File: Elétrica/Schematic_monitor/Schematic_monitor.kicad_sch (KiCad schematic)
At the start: 59 parts, among them J1 Conn_01x04, J2 USB_B_Micro, J3 Eletrode 1, J4 Eletrode 2, J5 Conn_01x09, SW1 SW_Push, SW2 SW_SPDT, U1 STM32F446RET6TR, U2 LM1117S-3.3, U3 MLX90614ESF-ACC-000-TU, U4 MAX30100EFD+, U5 AD623, U6 LM358, U7 LM358, U8 LM358, Y1 Crystal_25MHz

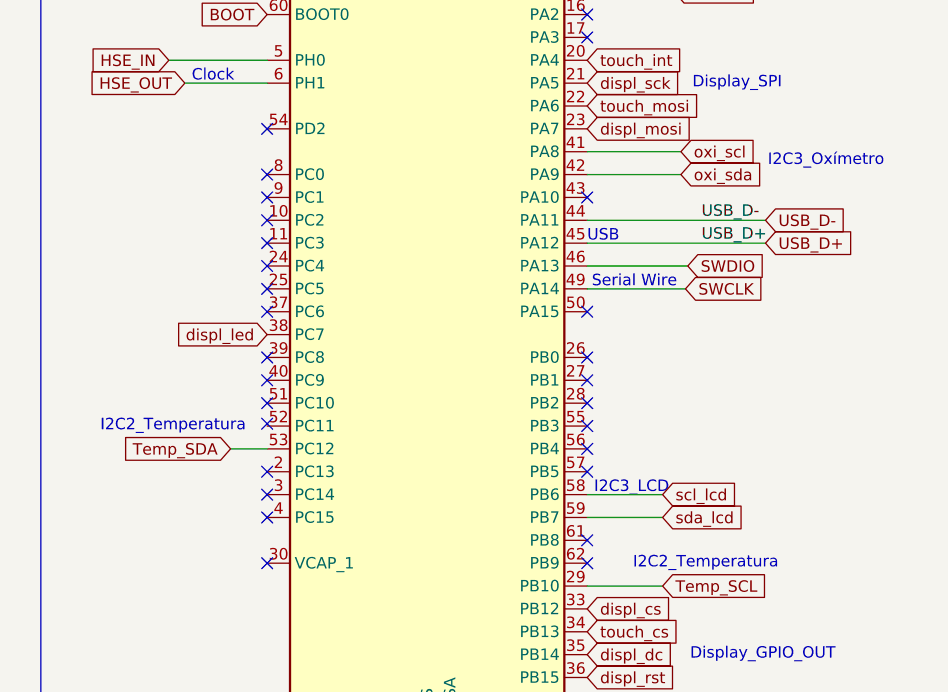
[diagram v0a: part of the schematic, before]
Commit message: Mudanças kicad
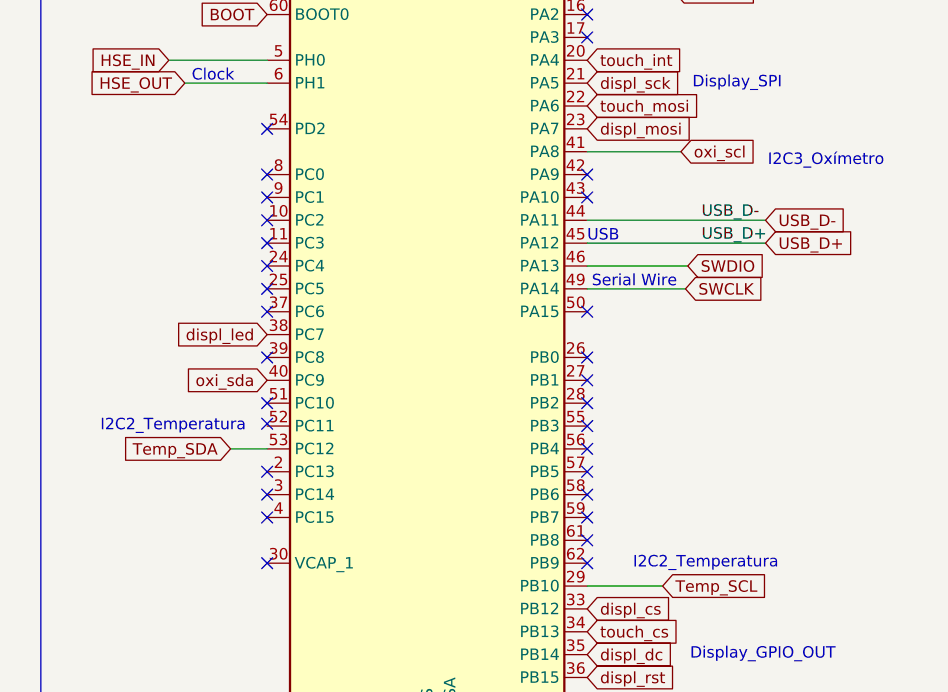
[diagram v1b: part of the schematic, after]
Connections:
- net oxi_sda: now also U1.40 (PC9); no longer U1.42 (PA9)
- net scl_lcd: no longer names the net of U1.58 (PB6)
- net sda_lcd: no longer names the net of U1.59 (PB7)
- no-connect marks 46 -> 48
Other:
- note removed: "I2C3_LCD"
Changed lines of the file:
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@@
   (no_connect (at 176.784 74.168))
   (no_connect (at 202.946 191.262))
+  (no_connect (at 238.506 201.422))
   (no_connect (at 238.506 148.082))
   (no_connect (at 202.946 201.422))
@@
   (no_connect (at 202.946 173.482))
   (no_connect (at 202.946 176.022))
+  (no_connect (at 238.506 203.962))
   (no_connect (at 238.506 181.102))
   (no_connect (at 202.946 198.882))
@@
   (no_connect (at 238.506 168.402))
   (no_connect (at 202.946 209.042))
-  (no_connect (at 202.946 188.722))
   (no_connect (at 77.47 148.59))
   (no_connect (at 238.506 191.262))
@@
   (no_connect (at 238.506 143.002))
   (no_connect (at 26.67 161.29))
+  (no_connect (at 238.506 165.862))
   (no_connect (at 160.274 64.008))
   (wire (pts (xy 119.888 118.364) (xy 119.888 122.428))
@@
     (stroke (width 0) (type default))
   )
-  (wire (pts (xy 238.506 201.422) (xy 246.888 201.422))
-    (stroke (width 0) (type default))
-  )
-  (wire (pts (xy 246.888 203.962) (xy 238.506 203.962))
-    (stroke (width 0) (type default))
-  )
   (wire (pts (xy 46.736 103.886) (xy 58.166 103.886))
     (stroke (width 0) (type default))
@@
   )
   (wire (pts (xy 238.506 145.542) (xy 248.158 145.542))
-    (stroke (width 0) (type default))
-  )
-  (wire (pts (xy 238.506 165.862) (xy 248.92 165.862))
     (stroke (width 0) (type default))
   )
@@
     (effects (font (size 1.27 1.27)) (justify left bottom))
   )
-  (text "I2C3_LCD\n" (at 239.268 201.422 0)
-    (effects (font (size 1.27 1.27)) (justify left bottom))
-  )
   (text "Fonte de Alimentação\n" (at 132.334 23.368 0)
     (effects (font (size 1.27 1.27)) (justify left bottom))
@@
     )
   )
-  (global_label "sda_lcd" (shape input) (at 246.888 203.962 0) (fields_autoplaced)
-    (effects (font (size 1.27 1.27)) (justify left))
-    (property "Intersheetrefs" "${INTERSHEET_REFS}" (at 256.9903 203.962 0)
-      (effects (font (size 1.27 1.27)) (justify left) hide)
-    )
-  )
   (global_label "displ_rst" (shape input) (at 170.434 106.68 0) (fields_autoplaced)
     (effects (font (size 1.27 1.27)) (justify left))
@@
     )
   )
-  (global_label "oxi_sda" (shape input) (at 248.92 165.862 0) (fields_autoplaced)
-    (effects (font (size 1.27 1.27)) (justify left))
-    (property "Intersheetrefs" "${INTERSHEET_REFS}" (at 258.9014 165.862 0)
-      (effects (font (size 1.27 1.27)) (justify left) hide)
-    )
-  )
   (global_label "displ_sck" (shape input) (at 238.506 155.702 0) (fields_autoplaced)
     (effects (font (size 1.27 1.27)) (justify left))
@@
     )
   )
+  (global_label "oxi_sda" (shape input) (at 202.946 188.722 180) (fields_autoplaced)
+    (effects (font (size 1.27 1.27)) (justify right))
+    (property "Intersheetrefs" "${INTERSHEET_REFS}" (at 192.9646 188.722 0)
+      (effects (font (size 1.27 1.27)) (justify right) hide)
+    )
+  )
   (global_label "HSE_OUT" (shape input) (at 123.698 106.172 0) (fields_autoplaced)
     (effects (font (size 1.27 1.27)) (justify left))
@@
     )
   )
-  (global_label "scl_lcd" (shape input) (at 246.888 201.422 0) (fields_autoplaced)
-    (effects (font (size 1.27 1.27)) (justify left))
-    (property "Intersheetrefs" "${INTERSHEET_REFS}" (at 256.4461 201.422 0)
-      (effects (font (size 1.27 1.27)) (justify left) hide)
-    )
-  )

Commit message: Ajustes
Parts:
- D4: footprint Diode_SMD:D_SMB -> Diode_SMD:D_0603_1608Metric_Pad1.05x0.95mm_HandSolder
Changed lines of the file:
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@@
       (effects (font (size 1.27 1.27)) (justify left) hide)
     )
-    (property "Footprint" "Diode_SMD:D_SMB" (at 74.168 75.438 0)
+    (property "Footprint" "Diode_SMD:D_0603_1608Metric_Pad1.05x0.95mm_HandSolder" (at 74.168 75.438 0)
       (effects (font (size 1.27 1.27)) hide)
     )
@@
       (effects (font (size 1.27 1.27)) (justify left) hide)
     )
-    (property "Footprint" "Diode_SMD:D_SMB" (at 84.582 36.576 0)
-      (effects (font (size 1.27 1.27)) hide)
-    )
+    (property "Footprint" "Diode_SMD:D_0603_1608Metric_Pad1.05x0.95mm_HandSolder" (at 84.582 36.576 0)
+      (effects (font (size 1.27 1.27)) hide)
+    )

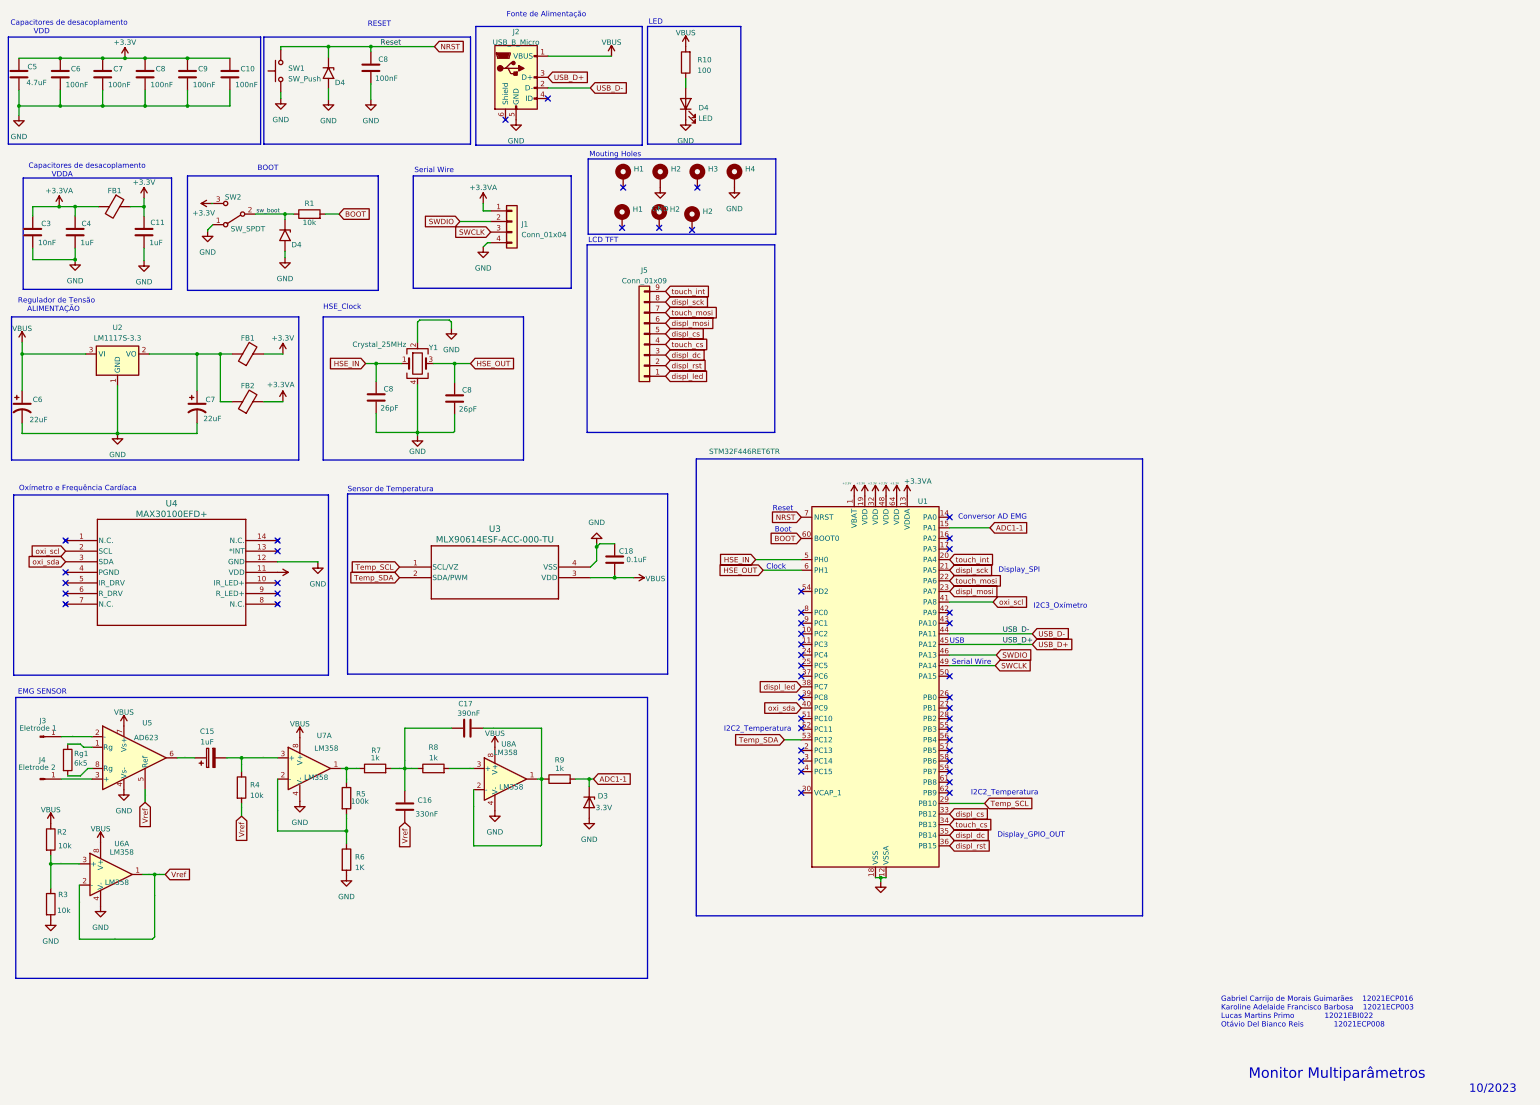
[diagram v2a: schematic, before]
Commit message: Inicio PRJ4
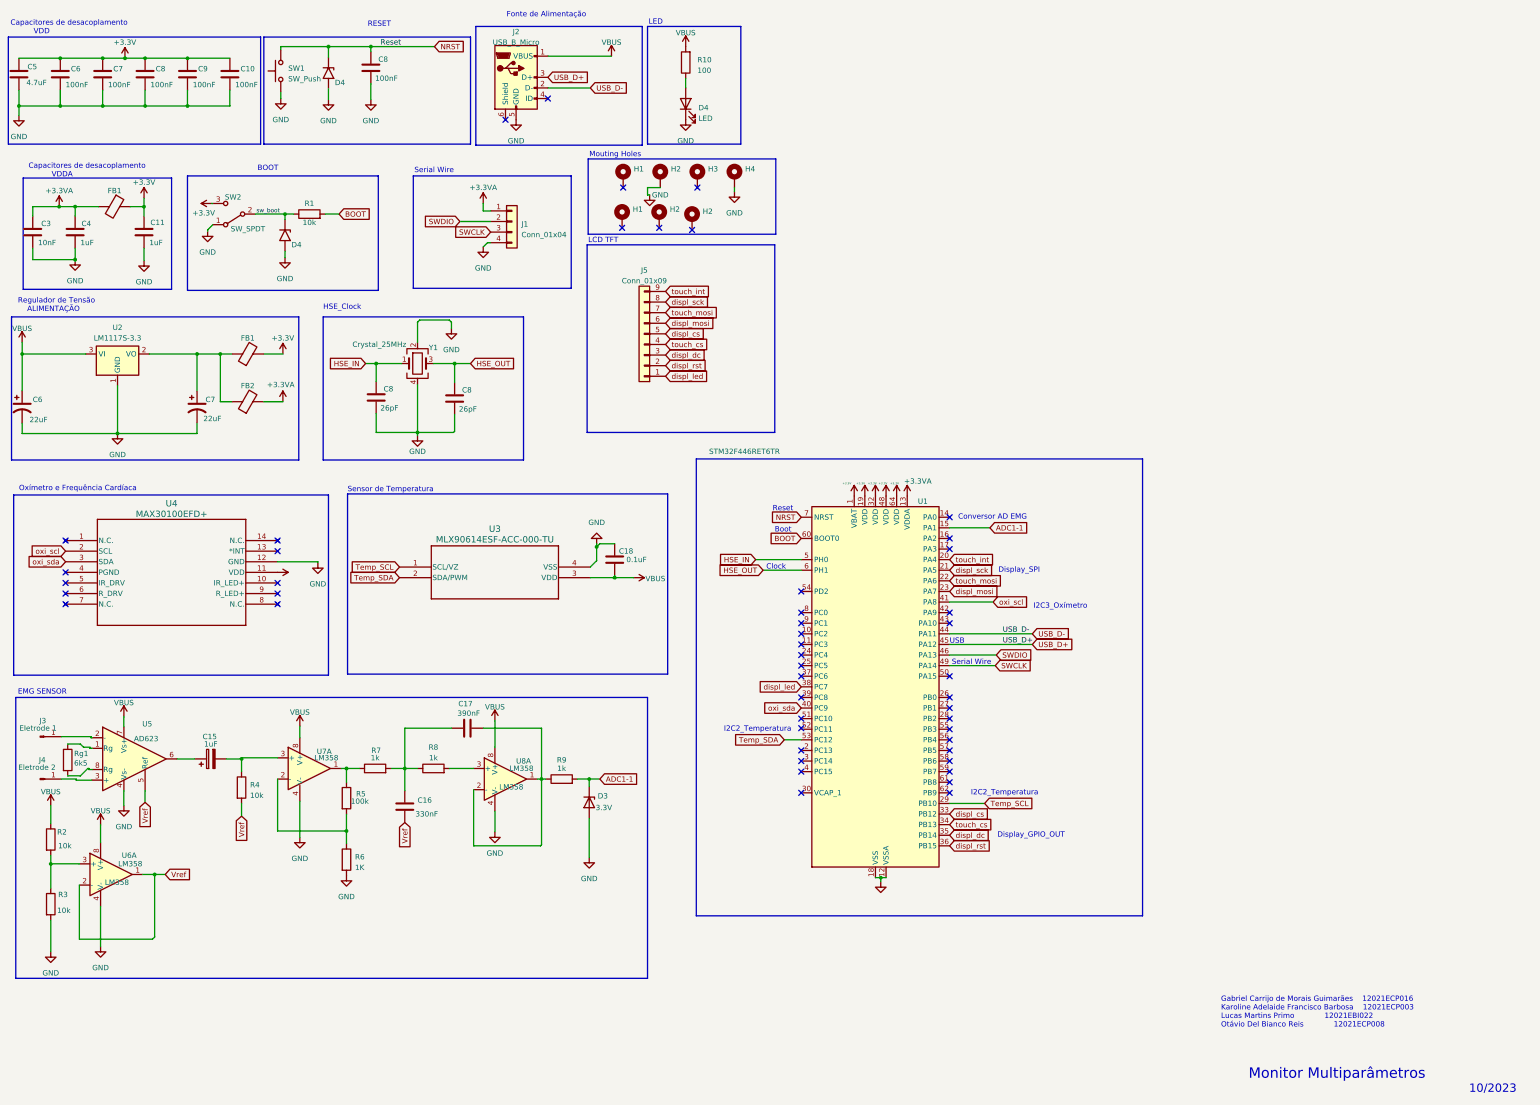
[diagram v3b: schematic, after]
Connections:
- net ADC1-1: no longer C15.1, C15.2, C16.1, C16.2, C17.1, C17.2, J3.1 (Pin_1), J4.1 (Pin_1), R2.2, R3.1, R4.1, R4.2, R5.1, R5.2, R6.1, R7.1, R7.2, R8.1, R8.2, R9.1, Rg1.1, U5.1 (Rg), U5.2 (-), U5.3 (+), U5.5 (Ref), U5.6, U6.1, U6.2 (-), U6.3 (+), U7.1, U7.2 (-), U7.3 (+), U8.1, U8.2 (-), U8.3 (+)
- new net: C16.1, C17.1, R7.2, R8.1
- new net: R8.2, U8.3 (+)
- new net: C17.2, R9.1, U8.1, U8.2 (-)
- new net: J3.1 (Pin_1), U5.2 (-)
- new net: C15.2, R4.1, U7.3 (+)
- new net: J4.1 (Pin_1), U5.3 (+)
- new net: R5.1, R7.1, U7.1
- new net: R5.2, R6.1, U7.2 (-)
- new net: Rg1.1, U5.1 (Rg)
- new net: C15.1, U5.6
- new net: R2.2, R3.1, U6.3 (+)
- new net Vref: C16.2, R4.2, U5.5 (Ref), U6.1, U6.2 (-)
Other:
- moved on the sheet: R9

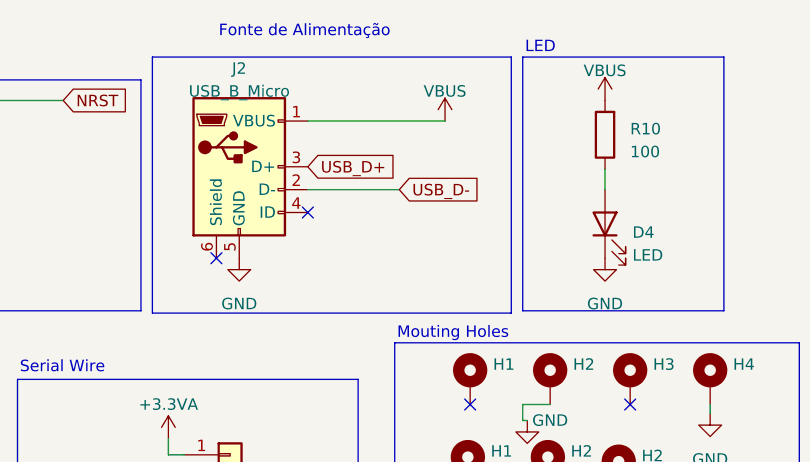
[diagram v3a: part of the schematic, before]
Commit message: PRJ4
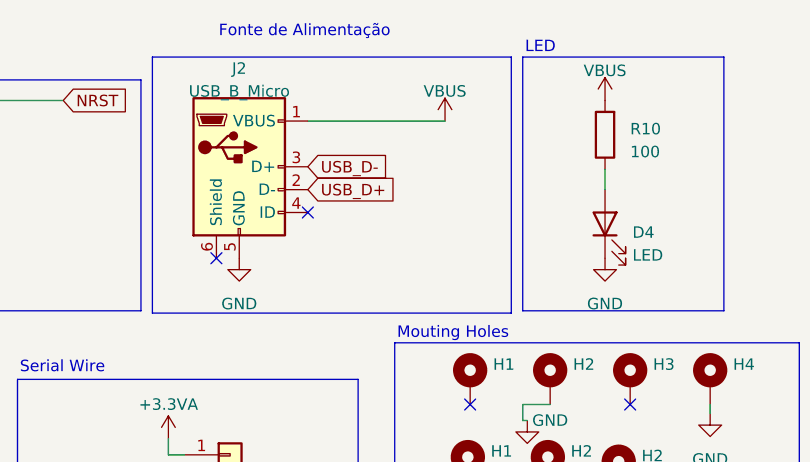
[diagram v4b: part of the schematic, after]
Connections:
- net USB_D+: now also J2.2 (D-); no longer J2.3 (D+)
- net USB_D-: now also J2.3 (D+); no longer J2.2 (D-)
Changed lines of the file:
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@@
-    (stroke (width 0) (type default))
-  )
-  (wire (pts (xy 152.4 40.132) (xy 142.24 40.132))
     (stroke (width 0) (type default))
   )
@@
     )
   )
-  (global_label "USB_D-" (shape input) (at 152.4 40.132 0) (fields_autoplaced)
-    (effects (font (size 1.27 1.27)) (justify left))
-    (property "Intersheetrefs" "${INTERSHEET_REFS}" (at 162.9258 40.132 0)
+  (global_label "USB_D-" (shape input) (at 142.24 37.592 0) (fields_autoplaced)
+    (effects (font (size 1.27 1.27)) (justify left))
+    (property "Intersheetrefs" "${INTERSHEET_REFS}" (at 152.7658 37.592 0)
       (effects (font (size 1.27 1.27)) (justify left) hide)
     )
@@
     )
   )
-  (global_label "USB_D+" (shape input) (at 142.24 37.592 0) (fields_autoplaced)
-    (effects (font (size 1.27 1.27)) (justify left))
-    (property "Intersheetrefs" "${INTERSHEET_REFS}" (at 152.7658 37.592 0)
-      (effects (font (size 1.27 1.27)) (justify left) hide)
-    )
+  (global_label "USB_D+" (shape input) (at 142.24 40.132 0) (fields_autoplaced)
+    (effects (font (size 1.27 1.27)) (justify left))
+    (property "Intersheetrefs" "${INTERSHEET_REFS}" (at 152.7658 40.132 0)
+      (effects (font (size 1.27 1.27)) (justify left) hide)
+    )
